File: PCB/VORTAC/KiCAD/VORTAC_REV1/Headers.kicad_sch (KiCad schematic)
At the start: 9 parts, among them J1 DEBUG, J14 918-418K2023S40001, J15 STEPPER, J3 Conn_02x02_Odd_Even

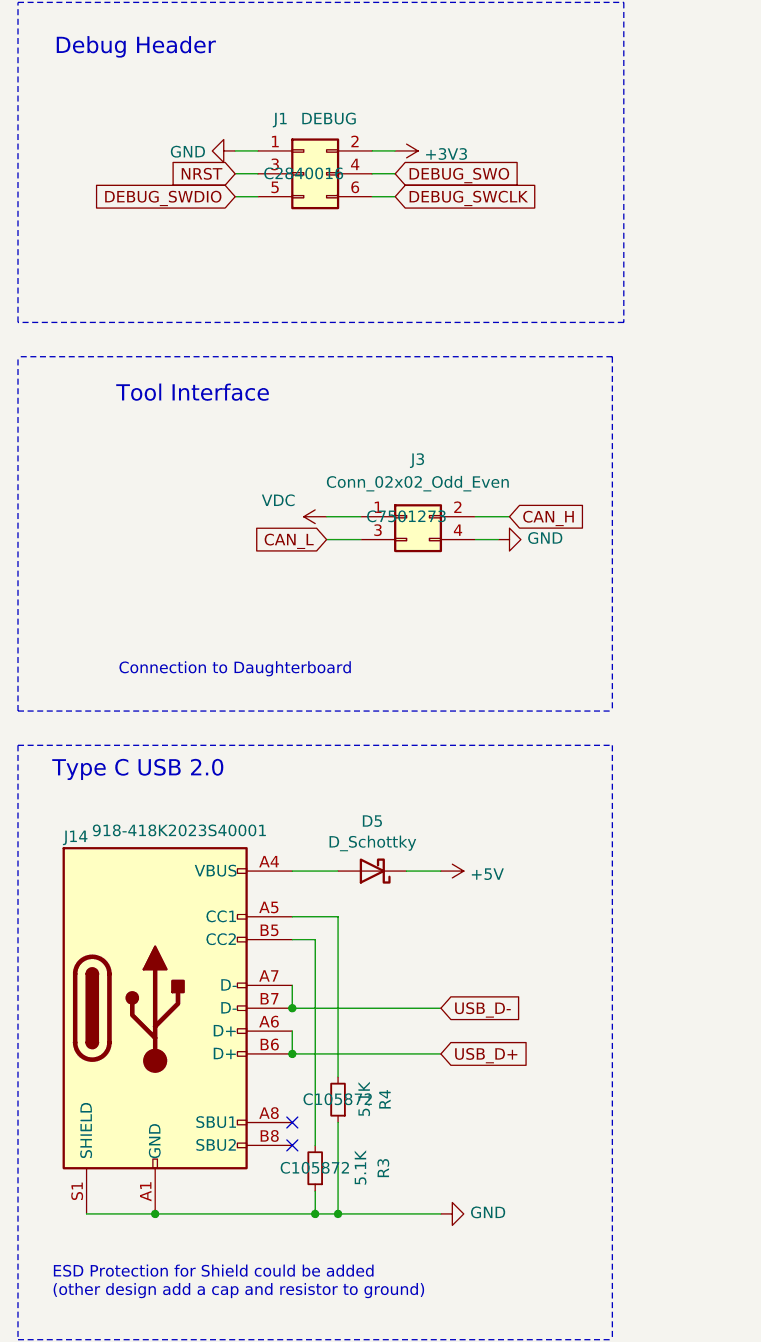
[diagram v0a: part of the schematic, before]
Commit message: Evil Mita is v00:98
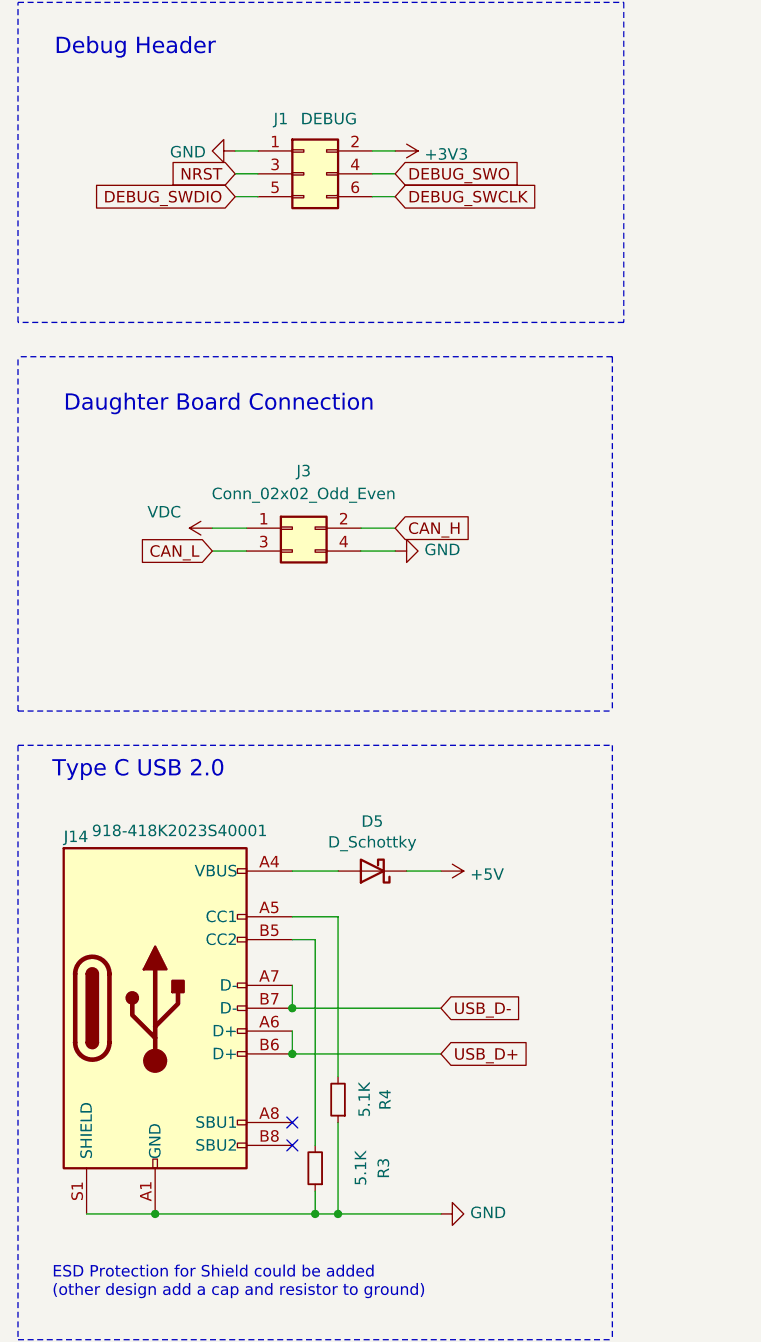
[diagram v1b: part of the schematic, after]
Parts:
- J1: LCSC C2840016 -> C541853
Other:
- note added: "Daughter Board Connection"
- note removed: "Connection to Daughterboard"
- note removed: "Tool Interface"
- moved on the sheet: J3
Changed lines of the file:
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@@
 		)
 	)
-	(text "Connection to Daughterboard"
-		(exclude_from_sim no)
-		(at 27.686 119.38 0)
-		(effects
-			(font
-				(size 1.27 1.27)
-			)
-			(justify left bottom)
-		)
-	)
-	(text "Tool Interface"
-		(exclude_from_sim no)
-		(at 27.432 89.154 0)
+	(text "Daughter Board Connection"
+		(exclude_from_sim no)
+		(at 21.59 90.17 0)
 		(effects
 			(font
@@
 	(wire
 		(pts
-			(xy 50.8 104.14) (xy 54.61 104.14)
+			(xy 38.1 105.41) (xy 41.91 105.41)
 		)
 		(stroke
@@
 	(wire
 		(pts
-			(xy 71.12 101.6) (xy 67.31 101.6)
+			(xy 58.42 102.87) (xy 54.61 102.87)
 		)
 		(stroke
@@
 	(wire
 		(pts
-			(xy 69.85 104.14) (xy 67.31 104.14)
+			(xy 58.42 105.41) (xy 54.61 105.41)
 		)
 		(stroke
@@
 	(wire
 		(pts
-			(xy 50.8 101.6) (xy 54.61 101.6)
+			(xy 38.1 102.87) (xy 41.91 102.87)
 		)
 		(stroke
@@
 	(global_label "CAN_L"
 		(shape input)
-		(at 50.8 104.14 180)
+		(at 38.1 105.41 180)
 		(effects
 			(font
@@
 		)
 		(property "Intersheetrefs" "${INTERSHEET_REFS}"
-			(at 50.8 104.14 0)
+			(at 38.1 105.41 0)
 			(effects
 				(font
@@
 	(global_label "CAN_H"
 		(shape input)
-		(at 71.12 101.6 0)
+		(at 58.42 102.87 0)
 		(effects
 			(font
@@
 		)
 		(property "Intersheetrefs" "${INTERSHEET_REFS}"
-			(at 71.12 101.6 0)
+			(at 58.42 102.87 0)
 			(effects
 				(font
@@
 					(size 1.27 1.27)
 				)
+				(hide yes)
 			)
 		)
@@
 					(size 1.27 1.27)
 				)
+				(hide yes)
 			)
 		)
@@
 			)
 		)
-		(property "LCSC" "C2840016"
+		(property "LCSC" "C541853"
 			(at 48.26 63.5 0)
 			(effects
@@
 					(size 1.27 1.27)
 				)
+				(hide yes)
 			)
 		)
@@
 	(symbol
 		(lib_id "power:GND")
-		(at 69.85 104.14 90)
+		(at 58.42 105.41 90)
 		(unit 1)
 		(exclude_from_sim no)
@@
 		(dnp no)
 		(property "Reference" "#PWR120"
-			(at 76.2 104.14 0)
+			(at 64.77 105.41 0)
 			(effects
 				(font
@@
 		)
 		(property "Value" "GND"
-			(at 73.1012 104.013 90)
+			(at 61.6712 105.283 90)
 			(effects
 				(font
@@
 		)
 		(property "Footprint" ""
-			(at 69.85 104.14 0)
+			(at 58.42 105.41 0)
 			(effects
 				(font
@@
 		)
 		(property "Datasheet" ""
-			(at 69.85 104.14 0)
+			(at 58.42 105.41 0)
 			(effects
 				(font
@@
 		)
 		(property "Description" "Power symbol creates a global label with name \"GND\" , ground"
-			(at 69.85 104.14 0)
+			(at 58.42 105.41 0)
 			(effects
 				(font
@@
 	(symbol
 		(lib_id "Connector_Generic:Conn_02x02_Odd_Even")
-		(at 59.69 101.6 0)
+		(at 46.99 102.87 0)
 		(unit 1)
 		(exclude_from_sim no)
@@
 		(fields_autoplaced yes)
 		(property "Reference" "J3"
-			(at 60.96 95.25 0)
+			(at 48.26 96.52 0)
 			(effects
 				(font
@@
 		)
 		(property "Value" "Conn_02x02_Odd_Even"
-			(at 60.96 97.79 0)
+			(at 48.26 99.06 0)
 			(effects
 				(font
@@
 		)
 		(property "Footprint" "Connector_PinHeader_2.54mm:PinHeader_2x02_P2.54mm_Vertical"
-			(at 59.69 101.6 0)
+			(at 46.99 102.87 0)
 			(effects
 				(font
@@
 		)
 		(property "Datasheet" "~"
-			(at 59.69 101.6 0)
+			(at 46.99 102.87 0)
 			(effects
 				(font
@@
 		)
 		(property "Description" "Generic connector, double row, 02x02, odd/even pin numbering scheme (row 1 odd numbers, row 2 even numbers), script generated (kicad-library-utils/schlib/autogen/connector/)"
-			(at 59.69 101.6 0)
+			(at 46.99 102.87 0)
 			(effects
 				(font
@@
 		)
 		(property "LCSC" "C7501273"
-			(at 59.69 101.6 0)
-			(effects
-				(font
-					(size 1.27 1.27)
-				)
+			(at 46.99 102.87 0)
+			(effects
+				(font
+					(size 1.27 1.27)
+				)
+				(hide yes)
 			)
 		)
@@
 	(symbol
 		(lib_id "power:VDC")
-		(at 50.8 101.6 90)
+		(at 38.1 102.87 90)
 		(unit 1)
 		(exclude_from_sim no)
@@
 		(dnp no)
 		(property "Reference" "#PWR1"
-			(at 54.61 101.6 0)
+			(at 41.91 102.87 0)
 			(effects
 				(font
@@
 		)
 		(property "Value" "VDC"
-			(at 45.466 99.822 90)
+			(at 32.766 101.092 90)
 			(effects
 				(font
@@
 		)
 		(property "Footprint" ""
-			(at 50.8 101.6 0)
+			(at 38.1 102.87 0)
 			(effects
 				(font
@@
 		)
 		(property "Datasheet" ""
-			(at 50.8 101.6 0)
+			(at 38.1 102.87 0)
 			(effects
 				(font
@@
 		)
 		(property "Description" "Power symbol creates a global label with name \"VDC\""
-			(at 50.8 101.6 0)
-			(effects
-				(font
+			(at 38.1 102.87 0)
+			(effects
+				(font

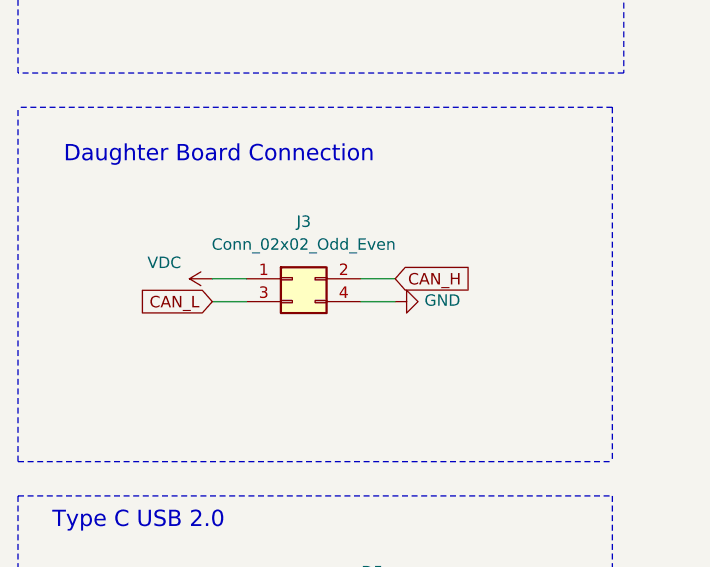
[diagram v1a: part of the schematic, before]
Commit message: No Body knows.... The trouble I've seen
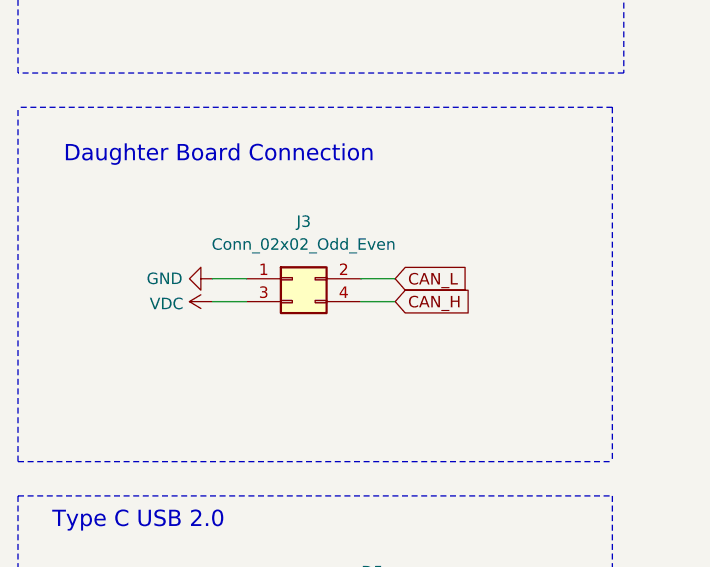
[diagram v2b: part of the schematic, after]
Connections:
- net CAN_H: now also J3.4 (Pin_4); no longer J3.2 (Pin_2)
- net CAN_L: now also J3.2 (Pin_2); no longer J3.3 (Pin_3)
- net GND: now also J3.1 (Pin_1); no longer J3.4 (Pin_4)
- net VDC: now also J3.3 (Pin_3); no longer J3.1 (Pin_1)
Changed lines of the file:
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@@
 	(global_label "CAN_L"
 		(shape input)
-		(at 38.1 105.41 180)
+		(at 58.42 102.87 0)
 		(effects
 			(font
 				(size 1.27 1.27)
 			)
-			(justify right)
+			(justify left)
 		)
 		(property "Intersheetrefs" "${INTERSHEET_REFS}"
-			(at 38.1 105.41 0)
+			(at 58.42 102.87 0)
 			(effects
 				(font
@@
 	(global_label "CAN_H"
 		(shape input)
-		(at 58.42 102.87 0)
+		(at 58.42 105.41 0)
 		(effects
 			(font
@@
 		)
 		(property "Intersheetrefs" "${INTERSHEET_REFS}"
-			(at 58.42 102.87 0)
+			(at 58.42 105.41 0)
 			(effects
 				(font
@@
 	(symbol
 		(lib_id "power:GND")
-		(at 58.42 105.41 90)
+		(at 38.1 102.87 270)
 		(unit 1)
 		(exclude_from_sim no)
@@
 		(dnp no)
 		(property "Reference" "#PWR120"
-			(at 64.77 105.41 0)
+			(at 31.75 102.87 0)
 			(effects
 				(font
@@
 		)
 		(property "Value" "GND"
-			(at 61.6712 105.283 90)
+			(at 34.798 102.87 90)
 			(effects
 				(font
@@
 		)
 		(property "Footprint" ""
-			(at 58.42 105.41 0)
+			(at 38.1 102.87 0)
 			(effects
 				(font
@@
 		)
 		(property "Datasheet" ""
-			(at 58.42 105.41 0)
+			(at 38.1 102.87 0)
 			(effects
 				(font
@@
 		)
 		(property "Description" "Power symbol creates a global label with name \"GND\" , ground"
-			(at 58.42 105.41 0)
+			(at 38.1 102.87 0)
 			(effects
 				(font
@@
 	(symbol
 		(lib_id "power:VDC")
-		(at 38.1 102.87 90)
+		(at 38.1 105.41 90)
 		(unit 1)
 		(exclude_from_sim no)
@@
 		(dnp no)
 		(property "Reference" "#PWR1"
-			(at 41.91 102.87 0)
+			(at 41.91 105.41 0)
 			(effects
 				(font
@@
 		)
 		(property "Value" "VDC"
-			(at 32.766 101.092 90)
+			(at 33.02 105.664 90)
 			(effects
 				(font
@@
 		)
 		(property "Footprint" ""
-			(at 38.1 102.87 0)
+			(at 38.1 105.41 0)
 			(effects
 				(font
@@
 		)
 		(property "Datasheet" ""
-			(at 38.1 102.87 0)
+			(at 38.1 105.41 0)
 			(effects
 				(font
@@
 		)
 		(property "Description" "Power symbol creates a global label with name \"VDC\""
-			(at 38.1 102.87 0)
-			(effects
-				(font
+			(at 38.1 105.41 0)
+			(effects
+				(font

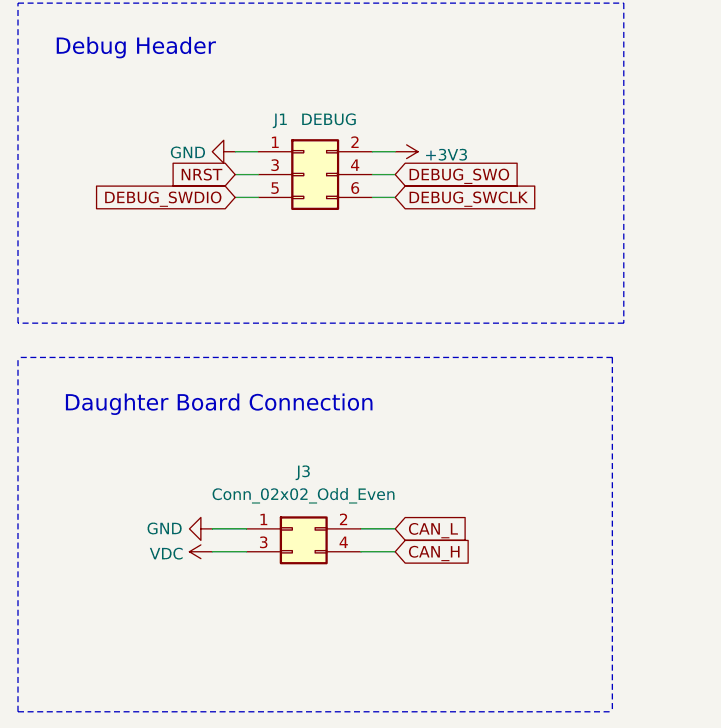
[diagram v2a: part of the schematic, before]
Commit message: Girl Math
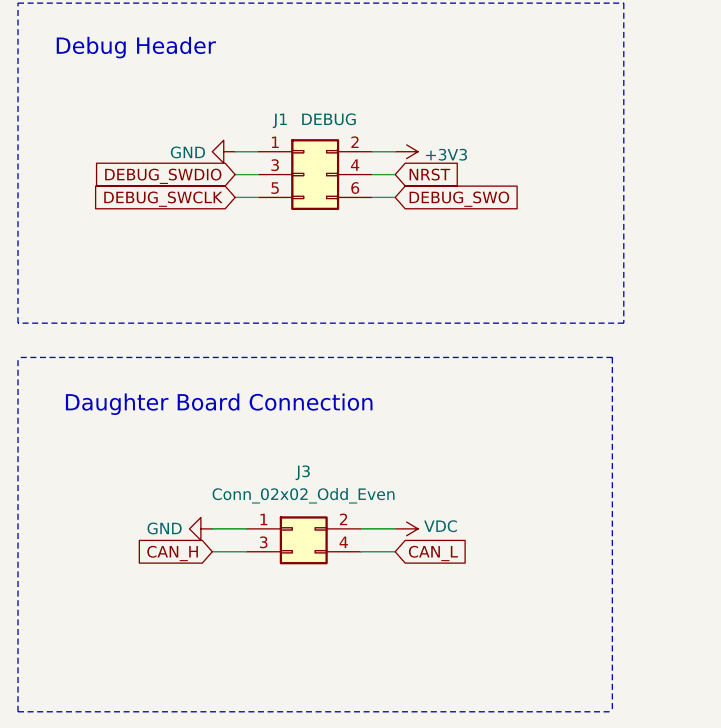
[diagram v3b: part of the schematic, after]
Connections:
- net CAN_H: now also J3.3 (Pin_3); no longer J3.4 (Pin_4)
- net CAN_L: now also J3.4 (Pin_4); no longer J3.2 (Pin_2)
- net DEBUG_SWCLK: now also J1.5 (Pin_5); no longer J1.6 (Pin_6)
- net DEBUG_SWDIO: now also J1.3 (Pin_3); no longer J1.5 (Pin_5)
- net DEBUG_SWO: now also J1.6 (Pin_6); no longer J1.4 (Pin_4)
- net NRST: now also J1.4 (Pin_4); no longer J1.3 (Pin_3)
- net VDC: now also J3.2 (Pin_2); no longer J3.3 (Pin_3)
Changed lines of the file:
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@@
 	(global_label "DEBUG_SWDIO"
 		(shape input)
-		(at 40.64 66.04 180)
+		(at 40.64 63.5 180)
 		(effects
 			(font
@@
 		)
 		(property "Intersheetrefs" "${INTERSHEET_REFS}"
-			(at 40.64 66.04 0)
+			(at 40.64 63.5 0)
 			(effects
 				(font
@@
 	(global_label "CAN_L"
 		(shape input)
-		(at 58.42 102.87 0)
+		(at 58.42 105.41 0)
 		(effects
 			(font
@@
 		)
 		(property "Intersheetrefs" "${INTERSHEET_REFS}"
-			(at 58.42 102.87 0)
+			(at 58.42 105.41 0)
 			(effects
 				(font
@@
 	(global_label "NRST"
 		(shape input)
-		(at 40.64 63.5 180)
-		(effects
-			(font
-				(size 1.27 1.27)
-			)
-			(justify right)
-		)
-		(property "Intersheetrefs" "${INTERSHEET_REFS}"
-			(at 40.64 63.5 0)
-			(effects
-				(font
-					(size 1.27 1.27)
-				)
-				(hide yes)
-			)
-		)
-	)
-	(global_label "DEBUG_SWO"
-		(shape input)
 		(at 58.42 63.5 0)
 		(effects
@@
 		)
 	)
-	(global_label "CAN_H"
-		(shape input)
-		(at 58.42 105.41 0)
-		(effects
-			(font
-				(size 1.27 1.27)
-			)
-			(justify left)
-		)
-		(property "Intersheetrefs" "${INTERSHEET_REFS}"
-			(at 58.42 105.41 0)
-			(effects
-				(font
-					(size 1.27 1.27)
-				)
-				(hide yes)
-			)
-		)
-	)
-	(global_label "DEBUG_SWCLK"
+	(global_label "DEBUG_SWO"
 		(shape input)
 		(at 58.42 66.04 0)
@@
 		)
 	)
+	(global_label "CAN_H"
+		(shape input)
+		(at 38.1 105.41 180)
+		(effects
+			(font
+				(size 1.27 1.27)
+			)
+			(justify right)
+		)
+		(property "Intersheetrefs" "${INTERSHEET_REFS}"
+			(at 38.1 105.41 0)
+			(effects
+				(font
+					(size 1.27 1.27)
+				)
+				(hide yes)
+			)
+		)
+	)
+	(global_label "DEBUG_SWCLK"
+		(shape input)
+		(at 40.64 66.04 180)
+		(effects
+			(font
+				(size 1.27 1.27)
+			)
+			(justify right)
+		)
+		(property "Intersheetrefs" "${INTERSHEET_REFS}"
+			(at 40.64 66.04 0)
+			(effects
+				(font
+					(size 1.27 1.27)
+				)
+				(hide yes)
+			)
+		)
+	)
 	(symbol
 		(lib_id "Connector_Generic:Conn_01x04")
@@
 	(symbol
 		(lib_id "power:VDC")
-		(at 38.1 105.41 90)
+		(at 58.42 102.87 270)
 		(unit 1)
 		(exclude_from_sim no)
@@
 		(dnp no)
 		(property "Reference" "#PWR1"
-			(at 41.91 105.41 0)
+			(at 54.61 102.87 0)
 			(effects
 				(font
@@
 		)
 		(property "Value" "VDC"
-			(at 33.02 105.664 90)
+			(at 63.5 102.616 90)
 			(effects
 				(font
@@
 		)
 		(property "Footprint" ""
-			(at 38.1 105.41 0)
+			(at 58.42 102.87 0)
 			(effects
 				(font
@@
 		)
 		(property "Datasheet" ""
-			(at 38.1 105.41 0)
+			(at 58.42 102.87 0)
 			(effects
 				(font
@@
 		)
 		(property "Description" "Power symbol creates a global label with name \"VDC\""
-			(at 38.1 105.41 0)
-			(effects
-				(font
+			(at 58.42 102.87 0)
+			(effects
+				(font
